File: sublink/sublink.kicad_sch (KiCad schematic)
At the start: 45 parts, among them J1 ZL315-4SGH, Q1 YJL2305A, SW1 SW_Push, SW2 SW_Push, SW3 SW_Push, U1 ATtiny414-SS, U2 OKY3402, U3 JS202011

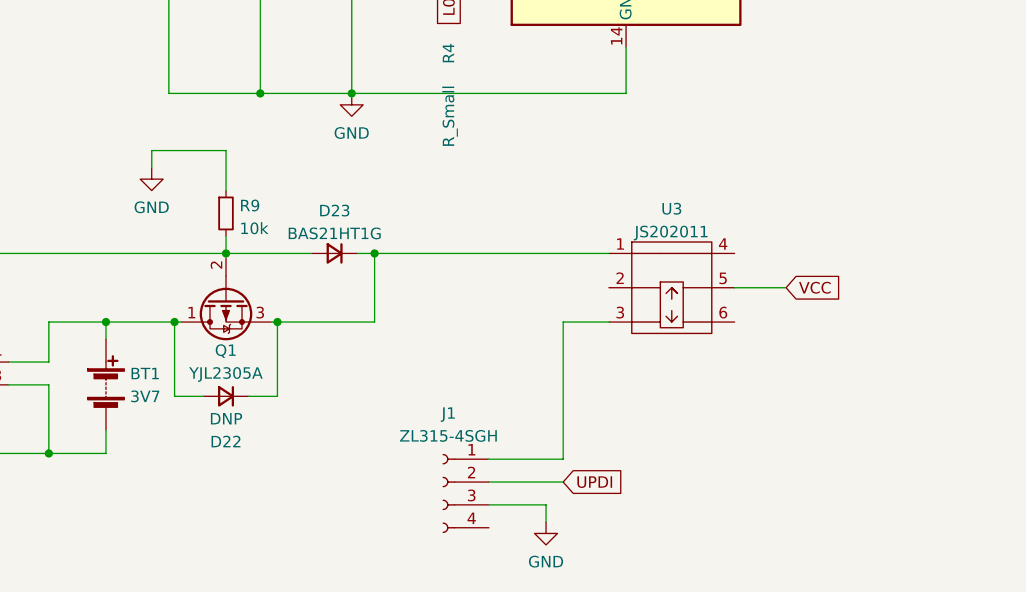
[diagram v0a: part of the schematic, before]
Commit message: wip routing
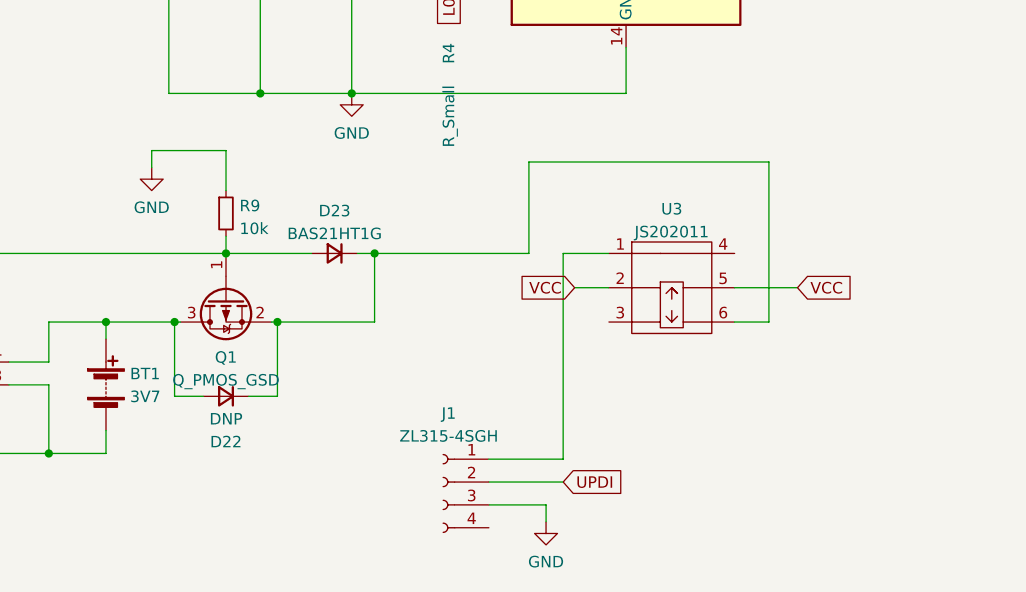
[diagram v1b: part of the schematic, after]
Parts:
- removed Q1: YJL2305A, Package_TO_SOT_SMD:SOT-23, symbol Device:Q_PMOS_DGS
- added Q1: Q_PMOS_GSD, Package_TO_SOT_SMD:SOT-23, symbol Device:Q_PMOS_GSD
- BT1: footprint Connector_PinHeader_2.54mm:PinHeader_1x02_P2.54mm_Vertical -> Resistor_SMD:R_1206_3216Metric_Pad1.30x1.75mm_HandSolder
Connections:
- net VCC: now also U3.2
- net at D23.2 (A), R9.2, U2.2 (USB+): now also Q1.1 (G)
- net at BT1.1 (+), D22.2 (A), U2.4 (B+): now also Q1.3 (D)
- net at D22.1 (K), D23.1 (K): now also U3.6, Q1.2 (S); no longer U3.1
- net at J1.1 (Pin_1): now also U3.1; no longer U3.3
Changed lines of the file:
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@@
   (junction (at 62.865 114.935) (diameter 0) (color 0 0 0 0)
   )
+  (junction (at 196.85 49.53) (diameter 0) (color 0 0 0 0)
+  )
   (junction (at 99.06 92.71) (diameter 0) (color 0 0 0 0)
   )
-  (junction (at 196.85 49.53) (diameter 0) (color 0 0 0 0)
-  )
   (junction (at 217.17 46.99) (diameter 0) (color 0 0 0 0)
   )
@@
     (stroke (width 0) (type default) (color 0 0 0 0))
   )
+  (wire (pts (xy 121.285 96.52) (xy 125.095 96.52))
+    (stroke (width 0) (type default) (color 0 0 0 0))
+  )
   (wire (pts (xy 62.865 114.935) (xy 69.215 114.935))
     (stroke (width 0) (type default) (color 0 0 0 0))
@@
     (stroke (width 0) (type default) (color 0 0 0 0))
   )
-  (wire (pts (xy 120.015 115.57) (xy 120.015 100.33))
-    (stroke (width 0) (type default) (color 0 0 0 0))
-  )
   (wire (pts (xy 86.36 62.23) (xy 86.36 74.93))
     (stroke (width 0) (type default) (color 0 0 0 0))
@@
     (stroke (width 0) (type default) (color 0 0 0 0))
   )
+  (wire (pts (xy 116.205 92.71) (xy 99.06 92.71))
+    (stroke (width 0) (type default) (color 0 0 0 0))
+  )
   (wire (pts (xy 207.01 41.91) (xy 207.01 55.88))
     (stroke (width 0) (type default) (color 0 0 0 0))
@@
     (stroke (width 0) (type default) (color 0 0 0 0))
   )
+  (wire (pts (xy 120.015 92.71) (xy 120.015 115.57))
+    (stroke (width 0) (type default) (color 0 0 0 0))
+  )
   (wire (pts (xy 214.63 46.99) (xy 217.17 46.99))
     (stroke (width 0) (type default) (color 0 0 0 0))
@@
     (stroke (width 0) (type default) (color 0 0 0 0))
   )
-  (wire (pts (xy 120.015 100.33) (xy 125.095 100.33))
-    (stroke (width 0) (type default) (color 0 0 0 0))
-  )
   (wire (pts (xy 217.17 39.37) (xy 217.17 41.91))
     (stroke (width 0) (type default) (color 0 0 0 0))
@@
     (stroke (width 0) (type default) (color 0 0 0 0))
   )
-  (wire (pts (xy 99.06 92.71) (xy 125.095 92.71))
+  (wire (pts (xy 116.205 82.55) (xy 116.205 92.71))
     (stroke (width 0) (type default) (color 0 0 0 0))
   )
@@
     (stroke (width 0) (type default) (color 0 0 0 0))
   )
+  (wire (pts (xy 142.875 82.55) (xy 116.205 82.55))
+    (stroke (width 0) (type default) (color 0 0 0 0))
+  )
   (wire (pts (xy 96.52 48.26) (xy 96.52 46.99))
     (stroke (width 0) (type default) (color 0 0 0 0))
@@
     (stroke (width 0) (type default) (color 0 0 0 0))
   )
-  (wire (pts (xy 139.065 96.52) (xy 144.78 96.52))
+  (wire (pts (xy 139.065 96.52) (xy 146.05 96.52))
     (stroke (width 0) (type default) (color 0 0 0 0))
   )
@@
     (stroke (width 0) (type default) (color 0 0 0 0))
   )
+  (wire (pts (xy 139.065 100.33) (xy 142.875 100.33))
+    (stroke (width 0) (type default) (color 0 0 0 0))
+  )
   (wire (pts (xy 186.69 55.88) (xy 193.04 55.88))
     (stroke (width 0) (type default) (color 0 0 0 0))
@@
     (stroke (width 0) (type default) (color 0 0 0 0))
   )
+  (wire (pts (xy 120.015 92.71) (xy 125.095 92.71))
+    (stroke (width 0) (type default) (color 0 0 0 0))
+  )
   (wire (pts (xy 214.63 41.91) (xy 217.17 41.91))
     (stroke (width 0) (type default) (color 0 0 0 0))
@@
   )
   (wire (pts (xy 176.53 39.37) (xy 179.07 39.37))
+    (stroke (width 0) (type default) (color 0 0 0 0))
+  )
+  (wire (pts (xy 142.875 82.55) (xy 142.875 100.33))
     (stroke (width 0) (type default) (color 0 0 0 0))
   )
@@
     )
   )
-  (global_label "VCC" (shape input) (at 144.78 96.52 0) (fields_autoplaced)
-    (effects (font (size 1.27 1.27)) (justify left))
-    (property "Intersheet References" "${INTERSHEET_REFS}" (id 0) (at 150.8217 96.4406 0)
+  (global_label "VCC" (shape input) (at 146.05 96.52 0) (fields_autoplaced)
+    (effects (font (size 1.27 1.27)) (justify left))
+    (property "Intersheet References" "${INTERSHEET_REFS}" (id 0) (at 152.0917 96.4406 0)
       (effects (font (size 1.27 1.27)) (justify left) hide)
     )
@@
     (property "Intersheet References" "${INTERSHEET_REFS}" (id 0) (at 126.9033 118.0306 0)
       (effects (font (size 1.27 1.27)) (justify left) hide)
+    )
+  )
+  (global_label "VCC" (shape input) (at 121.285 96.52 180) (fields_autoplaced)
+    (effects (font (size 1.27 1.27)) (justify right))
+    (property "Intersheet References" "${INTERSHEET_REFS}" (id 0) (at 115.2433 96.5994 0)
+      (effects (font (size 1.27 1.27)) (justify right) hide)
     )
   )
@@
       (effects (font (size 1.27 1.27)) (justify left))
     )
-    (property "Footprint" "Connector_PinHeader_2.54mm:PinHeader_1x02_P2.54mm_Vertical" (id 2) (at 69.215 105.791 90)
+    (property "Footprint" "Resistor_SMD:R_1206_3216Metric_Pad1.30x1.75mm_HandSolder" (id 2) (at 69.215 105.791 90)
       (effects (font (size 1.27 1.27)) hide)
     )
@@
     (pin "2")
   )
-  (symbol (lib_id "Device:Q_PMOS_DGS") (at 82.55 97.79 90) (mirror x) (unit 1)
-    (in_bom yes) (on_board yes)
-    (property "Reference" "Q1" (id 0) (at 82.55 103.505 90))
-    (property "Value" "YJL2305A" (id 1) (at 82.55 106.045 90))
+  (symbol (lib_id "Device:R_Small") (at 96.52 50.8 0) (unit 1)
+    (in_bom yes) (on_board yes) (fields_autoplaced)
+    (property "Reference" "R3" (id 0) (at 98.0186 49.9653 0)
+      (effects (font (size 1.27 1.27)) (justify left))
+    )
+    (property "Value" "R_Small" (id 1) (at 98.0186 52.5022 0)
+      (effects (font (size 1.27 1.27)) (justify left))
+    )
+    (property "Footprint" "Resistor_SMD:R_0805_2012Metric_Pad1.20x1.40mm_HandSolder" (id 2) (at 96.52 50.8 0)
+      (effects (font (size 1.27 1.27)) hide)
+    )
+    (property "Datasheet" "~" (id 3) (at 96.52 50.8 0)
+      (effects (font (size 1.27 1.27)) hide)
+    )
+    (pin "1")
+    (pin "2")
+  )
+  (symbol (lib_id "Device:Q_PMOS_GSD") (at 82.55 97.79 90) (mirror x) (unit 1)
+    (in_bom yes) (on_board yes) (fields_autoplaced)
+    (property "Reference" "Q1" (id 0) (at 82.55 104.2654 90))
+    (property "Value" "Q_PMOS_GSD" (id 1) (at 82.55 106.8023 90))
     (property "Footprint" "Package_TO_SOT_SMD:SOT-23" (id 2) (at 80.01 102.87 0)
       (effects (font (size 1.27 1.27)) hide)
@@
     (pin "2")
     (pin "3")
-  )
-  (symbol (lib_id "Device:R_Small") (at 96.52 50.8 0) (unit 1)
-    (in_bom yes) (on_board yes) (fields_autoplaced)
-    (property "Reference" "R3" (id 0) (at 98.0186 49.9653 0)
-      (effects (font (size 1.27 1.27)) (justify left))
-    )
-    (property "Value" "R_Small" (id 1) (at 98.0186 52.5022 0)
-      (effects (font (size 1.27 1.27)) (justify left))
-    )
-    (property "Footprint" "Resistor_SMD:R_0805_2012Metric_Pad1.20x1.40mm_HandSolder" (id 2) (at 96.52 50.8 0)
-      (effects (font (size 1.27 1.27)) hide)
-    )
-    (property "Datasheet" "~" (id 3) (at 96.52 50.8 0)
-      (effects (font (size 1.27 1.27)) hide)
-    )
-    (pin "1")
-    (pin "2")
   )
   (symbol (lib_id "Device:LED_Small") (at 212.09 41.91 180) (unit 1)
@@
     )
     (path "/49787c66-f49d-4a79-a51d-f0e535a60cc0"
-      (reference "BT1") (unit 1) (value "3V7") (footprint "Connector_PinHeader_2.54mm:PinHeader_1x02_P2.54mm_Vertical")
+      (reference "BT1") (unit 1) (value "3V7") (footprint "Resistor_SMD:R_1206_3216Metric_Pad1.30x1.75mm_HandSolder")
     )
     (path "/8a653a42-4334-4d27-9c26-7376a1c6c756"
@@
       (reference "J1") (unit 1) (value "ZL315-4SGH") (footprint "Connector_Harwin:Harwin_M20-89004xx_1x04_P2.54mm_Horizontal")
     )
-    (path "/aa0a099c-479d-4909-8f65-0af88e650102"
-      (reference "Q1") (unit 1) (value "YJL2305A") (footprint "Package_TO_SOT_SMD:SOT-23")
+    (path "/aef741e9-e229-4c8d-b8c3-21ad5f571a00"
+      (reference "Q1") (unit 1) (value "Q_PMOS_GSD") (footprint "Package_TO_SOT_SMD:SOT-23")
     )
     (path "/480cfc26-2c62-4bd8-bba1-ebc5c356850c"
